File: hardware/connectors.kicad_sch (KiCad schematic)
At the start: 8 parts, among them J1 USB-C_GCT_USB4145-03-0070-C, J2 FTSH-107-01-L-D-K, J3 POWER & CAN & SPI2, J4 PWM1, J5 PWM2, T12 TP_VBUS

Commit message: usbc changed, foots for electro cap and +5 lay
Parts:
- J1: footprint SamacSys_Parts:USB4145030230C -> Connector_USB:USB_C_Receptacle_GCT_USB4110; Mouser Price/Stock https://www.mouser.pl/ProductDetail/GCT/USB4145-03-0070-C?q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 -> https://www.mouser.pl/datasheet/2/837/GCT_USB4110_Product_D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
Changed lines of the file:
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@@
 			)
 		)
-		(property "Footprint" "SamacSys_Parts:USB4145030230C"
+		(property "Footprint" "Connector_USB:USB_C_Receptacle_GCT_USB4110"
 			(at 88.9 67.31 0)
 			(effects
@@
 			)
 		)
-		(property "Mouser Price/Stock" "https://www.mouser.pl/ProductDetail/GCT/USB4145-03-0070-C?qs=vvQtp7zwQdNoT6Ti9aciDw%3D%3D&srsltid=AfmBOoq0uP6vTzB2zbnWyQUamBuKb60wxEO7ZLPCh7hQgy-ny-YsYWrG"
+		(property "Mouser Price/Stock" "https://www.mouser.pl/datasheet/2/837/GCT_USB4110_Product_Drawing___20k_cycles-3455479.pdf"
 			(at 67.31 57.15 0)
 			(effects

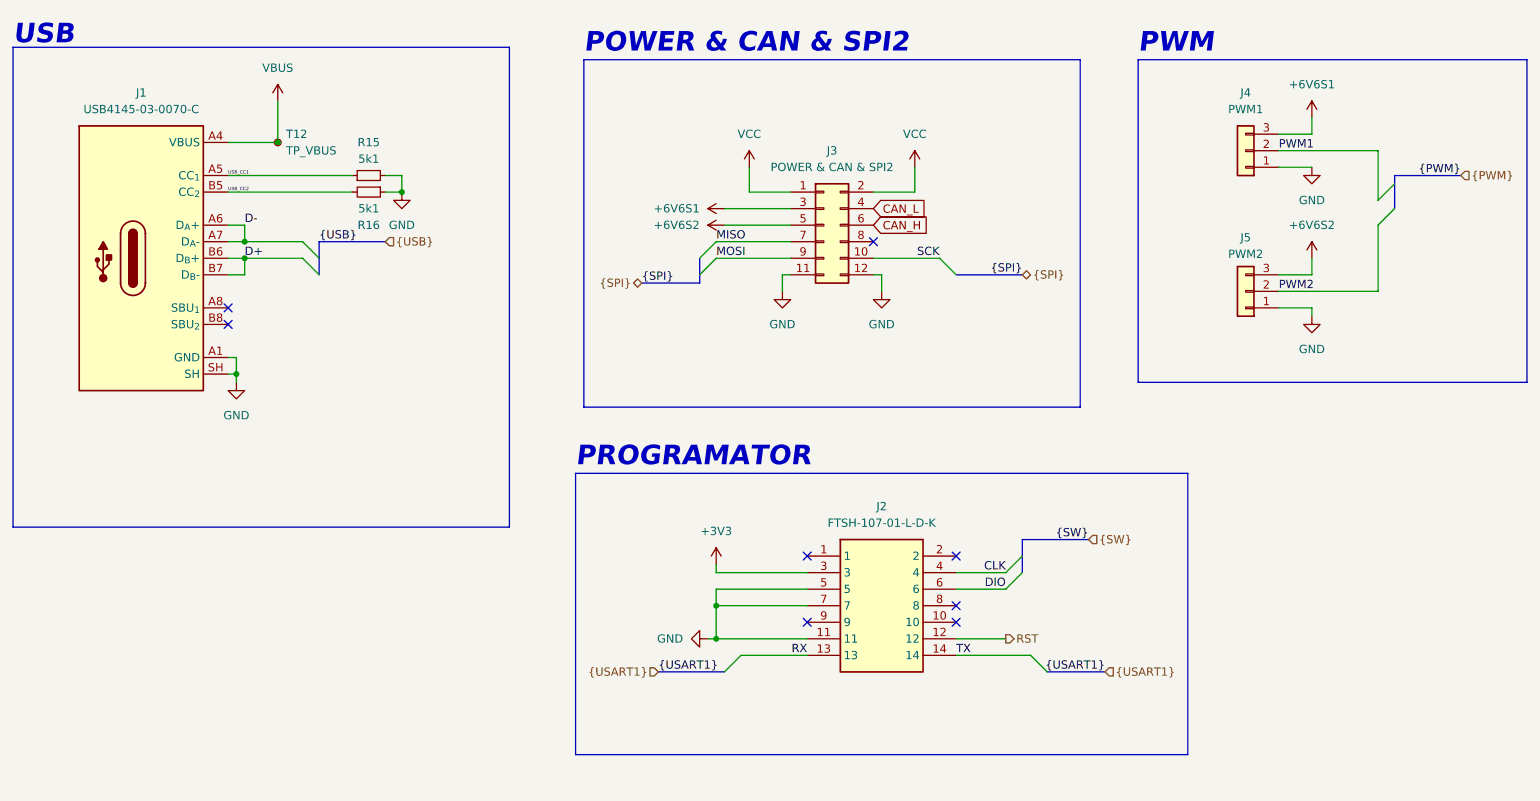
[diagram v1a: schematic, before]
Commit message: pcb & footprint update
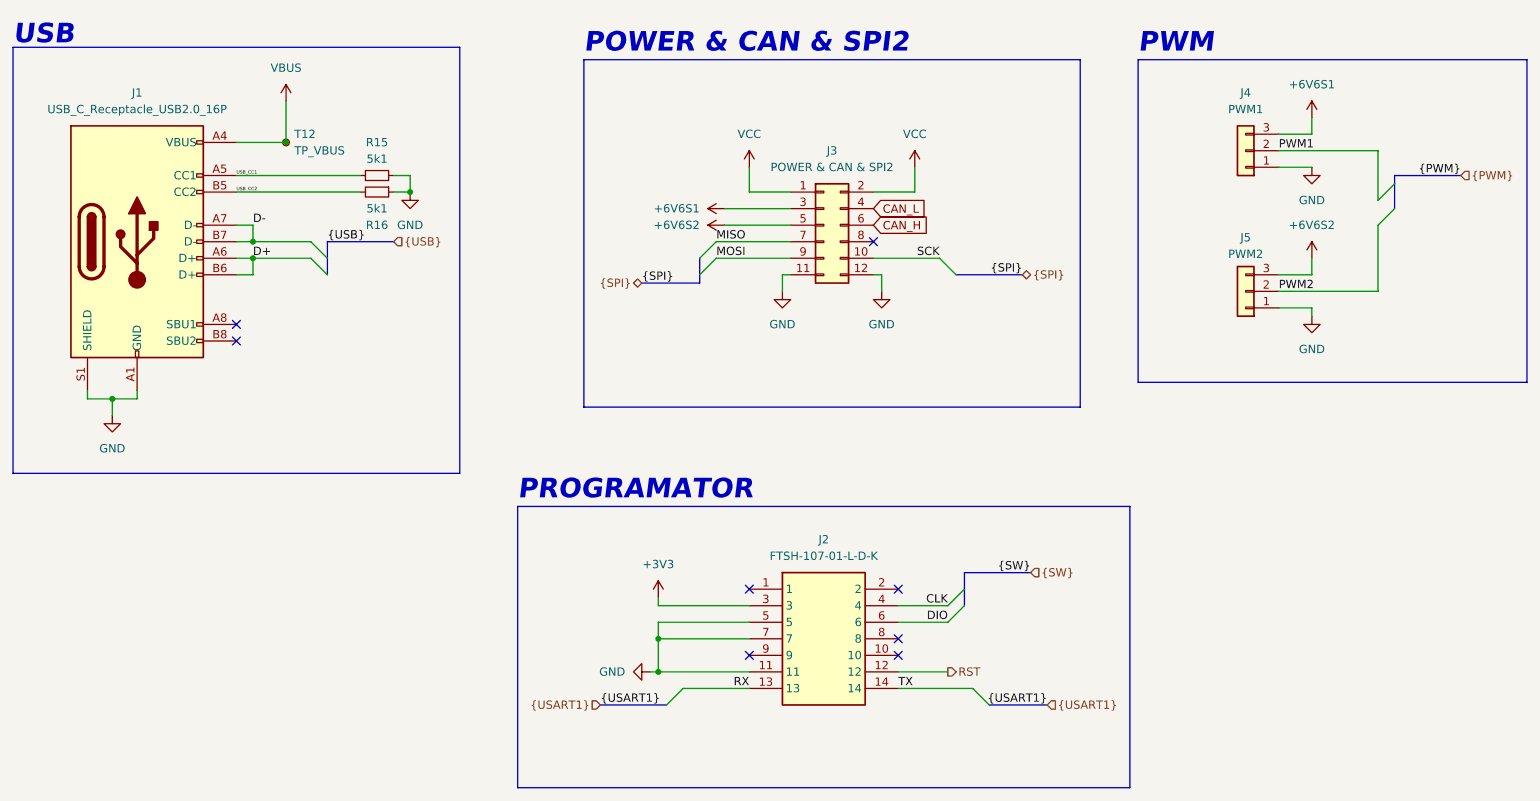
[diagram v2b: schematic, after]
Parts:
- removed J1: USB-C_GCT_USB4145-03-0070-C, Connector_USB:USB_C_Receptacle_GCT_USB4110, symbol USB-C_GCT_USB4145-03-0070-C:USB-C_GCT_USB4145-03-0070-C
- added J1: USB_C_Receptacle_USB2.0_16P, Connector_USB:USB_C_Receptacle_GCT_USB4105-xx-A_16P_TopMnt_Horizontal, symbol Connector:USB_C_Receptacle_USB2.0_16P
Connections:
- net D+: now also J1.A6 (D+), J1.B6 (D+)
- net D-: now also J1.A7 (D-), J1.B7 (D-)
- net GND: now also J1.A1 (GND), J1.A12 (GND), J1.B1 (GND), J1.B12 (GND), J1.S1 (SHIELD)
- net USB_CC1: now also J1.A5 (CC1)
- net USB_CC2: now also J1.B5 (CC2)
- net VBUS: now also J1.A4 (VBUS), J1.A9 (VBUS), J1.B4 (VBUS), J1.B9 (VBUS)
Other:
- moved on the sheet: J2, R15, R16, T12

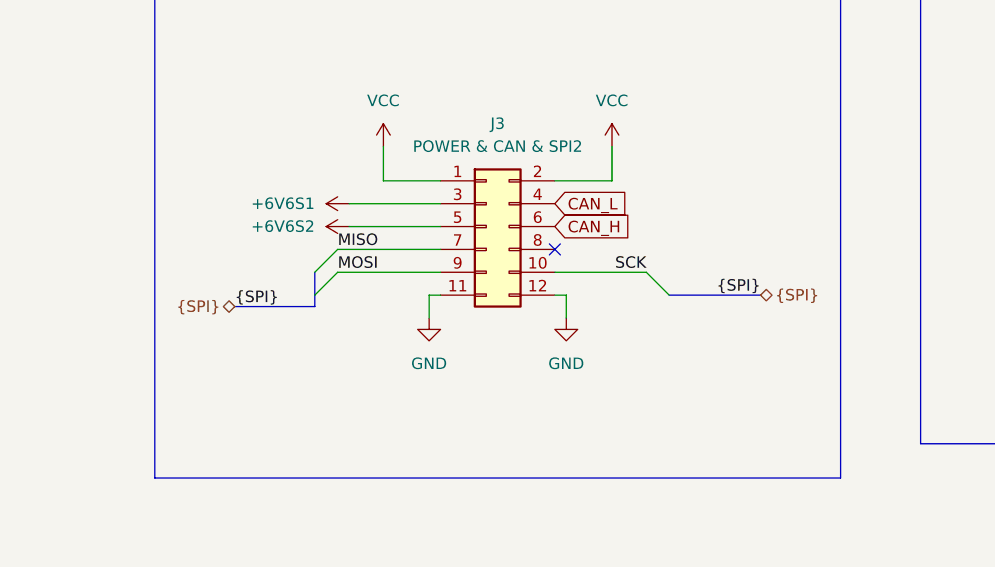
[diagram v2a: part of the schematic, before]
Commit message: pcb update
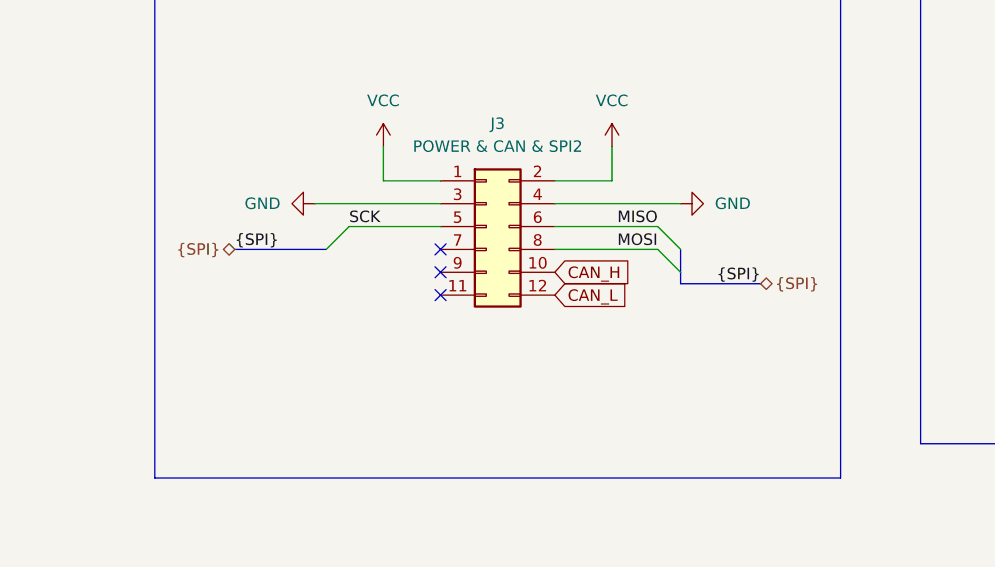
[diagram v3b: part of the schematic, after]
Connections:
- net +6V6S1: no longer J3.3 (Pin_3)
- net +6V6S2: no longer J3.5 (Pin_5)
- net CAN_H: now also J3.10 (Pin_10); no longer J3.6 (Pin_6)
- net CAN_L: now also J3.12 (Pin_12); no longer J3.4 (Pin_4)
- net GND: now also J3.3 (Pin_3), J3.4 (Pin_4); no longer J3.11 (Pin_11), J3.12 (Pin_12)
- net MISO: now also J3.6 (Pin_6); no longer J3.7 (Pin_7)
- net MOSI: now also J3.8 (Pin_8); no longer J3.9 (Pin_9)
- net SCK: now also J3.5 (Pin_5); no longer J3.10 (Pin_10)
- no-connect marks 8 -> 10

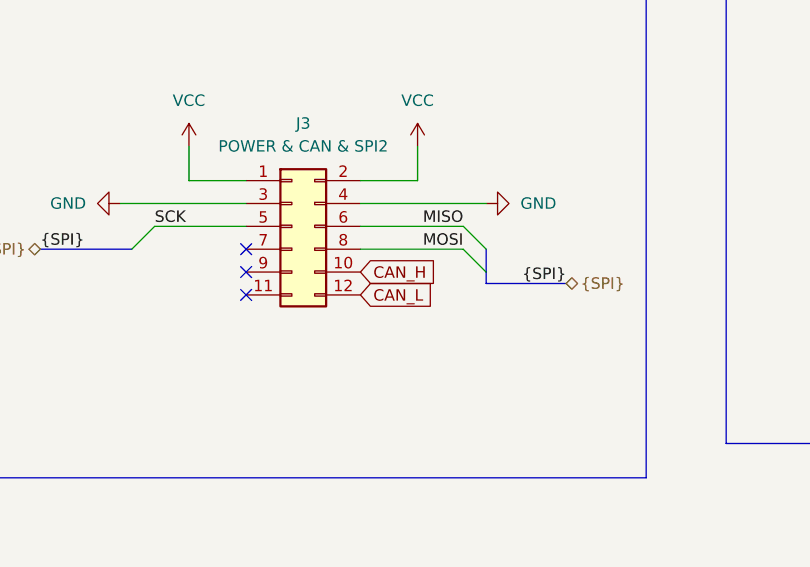
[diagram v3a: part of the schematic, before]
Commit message: pcb update
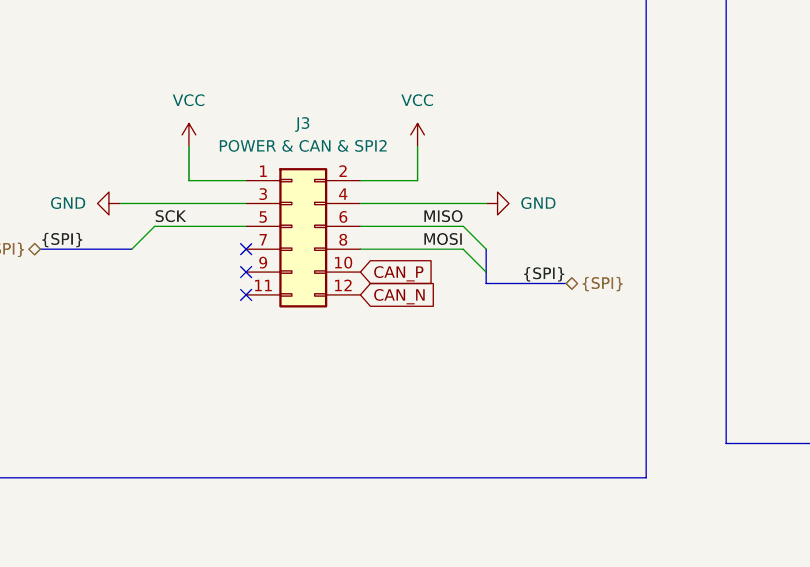
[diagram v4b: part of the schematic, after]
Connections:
- net CAN_H renamed CAN_P
- net CAN_L renamed CAN_N
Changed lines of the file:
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@@
 		)
 	)
-	(global_label "CAN_H"
+	(global_label "CAN_P"
 		(shape input)
 		(at 166.37 74.93 0)
@@
 		)
 		(property "Intersheetrefs" "${INTERSHEET_REFS}"
-			(at 175.3424 74.93 0)
+			(at 175.2819 74.93 0)
 			(effects
 				(font
@@
 		)
 	)
-	(global_label "CAN_L"
+	(global_label "CAN_N"
 		(shape input)
 		(at 166.37 77.47 0)
@@
 		)
 		(property "Intersheetrefs" "${INTERSHEET_REFS}"
-			(at 175.04 77.47 0)
+			(at 175.3424 77.47 0)
 			(effects
 				(font
